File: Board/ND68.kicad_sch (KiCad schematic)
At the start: 210 parts

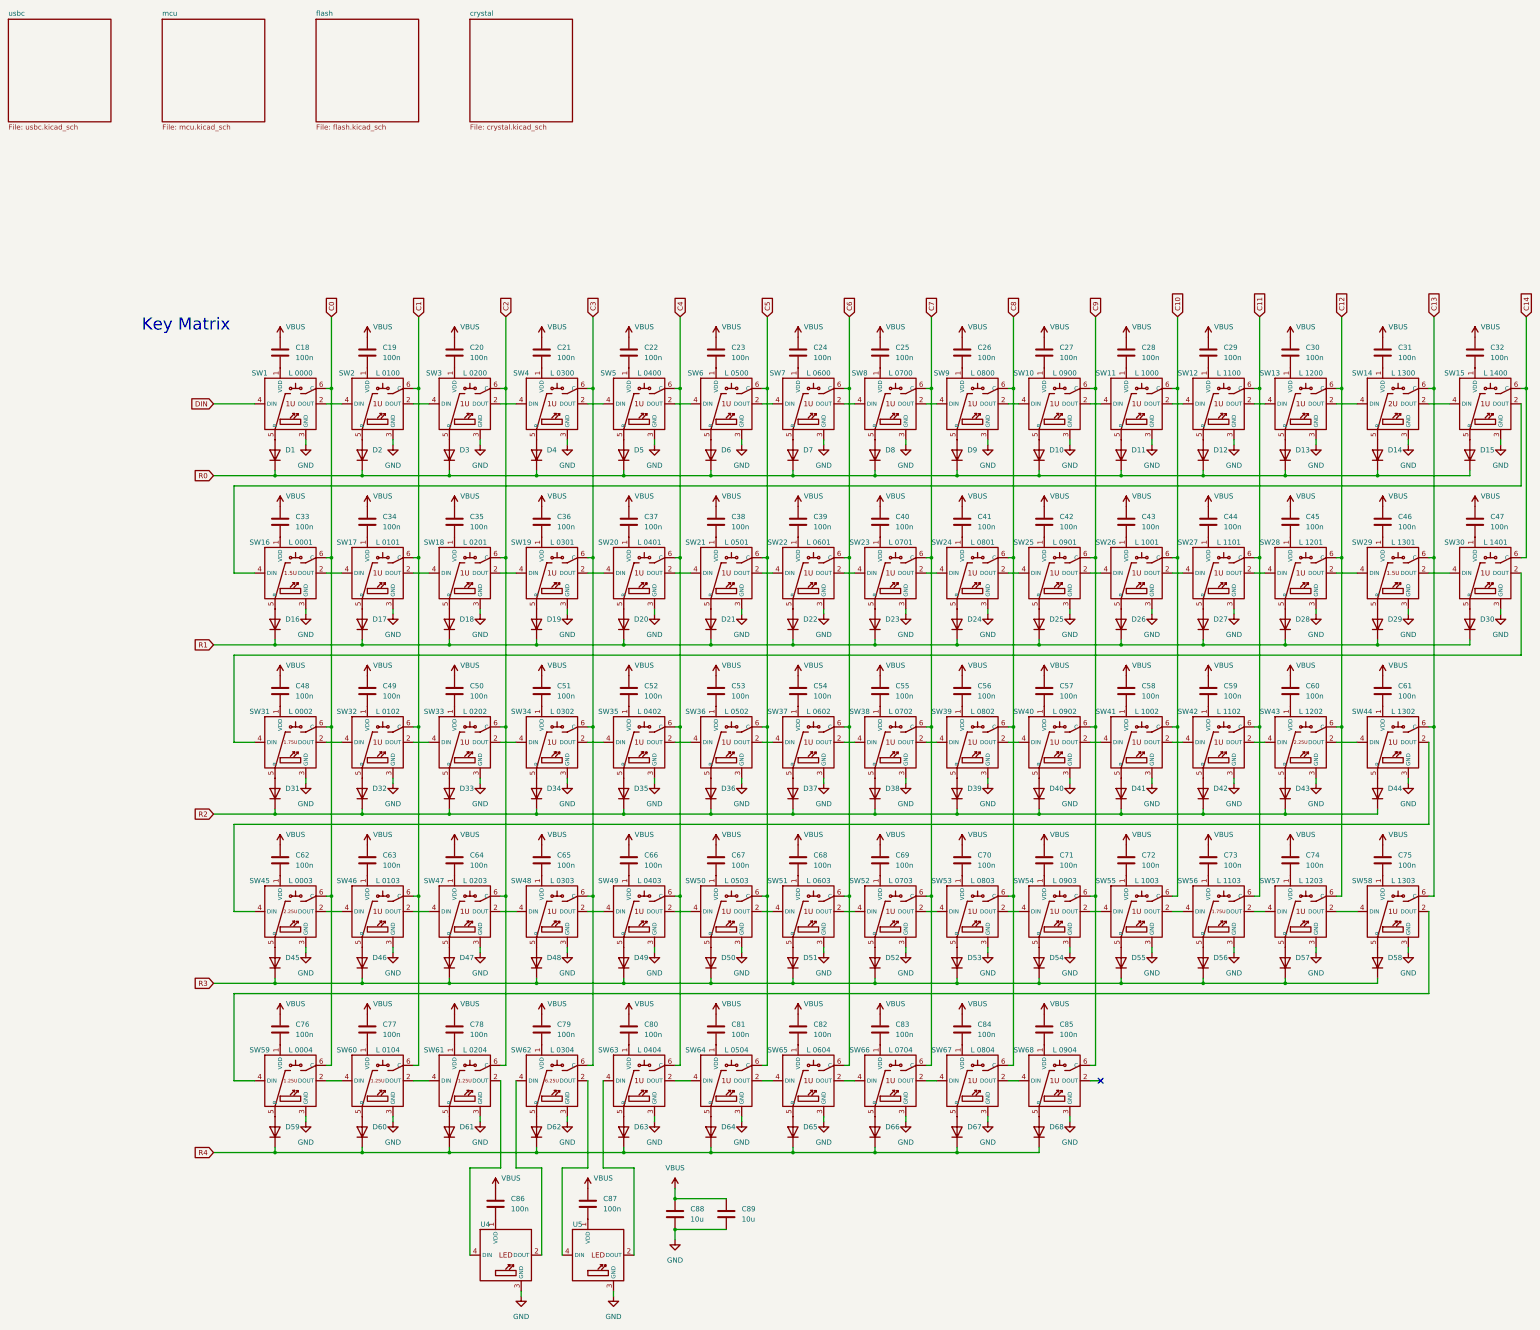
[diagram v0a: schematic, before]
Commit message: Rev 1 fix
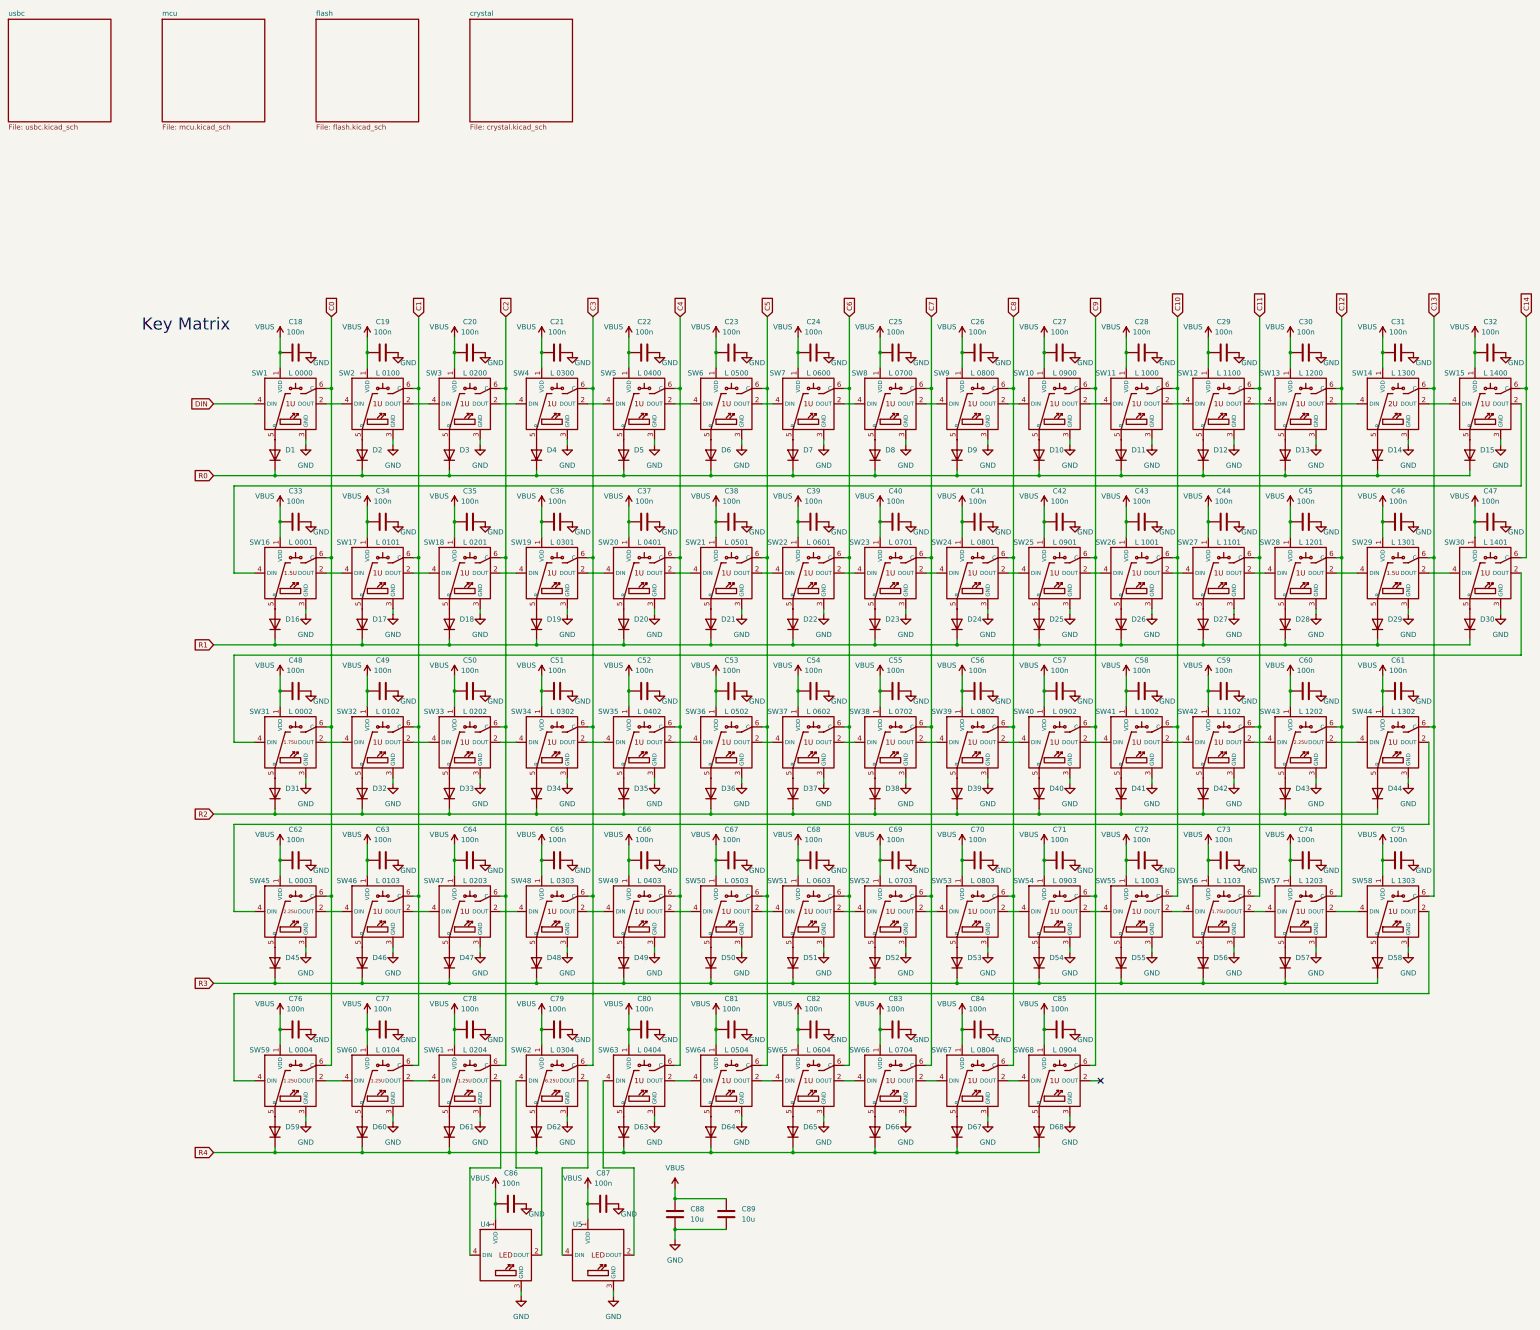
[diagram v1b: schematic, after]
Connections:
- net GND: now also C18.1, C19.2, C20.2, C21.2, C22.2, C23.2, C24.2, C25.2, C26.2, C27.2, C28.2, C29.2, C30.2, C31.2, C32.2, C33.2, C34.2, C35.2, C36.2, C37.2, C38.2, C39.2, C40.2, C41.2, C42.2, C43.2, C44.2, C45.2, C46.2, C47.2, C48.2, C49.2, C50.2, C51.2, C52.2, C53.2, C54.2, C55.2, C56.2, C57.2, C58.2, C59.2, C60.2, C61.2, C62.2, C63.2, C64.2, C65.2, C66.2, C67.2, C68.2, C69.2, C70.2, C71.2, C72.2, C73.2, C74.2, C75.2, C76.2, C77.2, C78.2, C79.2, C80.2, C81.2, C82.2, C83.2, C84.2, C85.2, C86.2, C87.2
- net VBUS: now also C18.2, SW1.1 (VDD), SW10.1 (VDD), SW11.1 (VDD), SW12.1 (VDD), SW13.1 (VDD), SW14.1 (VDD), SW15.1 (VDD), SW16.1 (VDD), SW17.1 (VDD), SW18.1 (VDD), SW19.1 (VDD), SW2.1 (VDD), SW20.1 (VDD), SW21.1 (VDD), SW22.1 (VDD), SW23.1 (VDD), SW24.1 (VDD), SW25.1 (VDD), SW26.1 (VDD), SW27.1 (VDD), SW28.1 (VDD), SW29.1 (VDD), SW3.1 (VDD), SW30.1 (VDD), SW31.1 (VDD), SW32.1 (VDD), SW33.1 (VDD), SW34.1 (VDD), SW35.1 (VDD), SW36.1 (VDD), SW37.1 (VDD), SW38.1 (VDD), SW39.1 (VDD), SW4.1 (VDD), SW40.1 (VDD), SW41.1 (VDD), SW42.1 (VDD), SW43.1 (VDD), SW44.1 (VDD), SW45.1 (VDD), SW46.1 (VDD), SW47.1 (VDD), SW48.1 (VDD), SW49.1 (VDD), SW5.1 (VDD), SW50.1 (VDD), SW51.1 (VDD), SW52.1 (VDD), SW53.1 (VDD), SW54.1 (VDD), SW55.1 (VDD), SW56.1 (VDD), SW57.1 (VDD), SW58.1 (VDD), SW59.1 (VDD), SW6.1 (VDD), SW60.1 (VDD), SW61.1 (VDD), SW62.1 (VDD), SW63.1 (VDD), SW64.1 (VDD), SW65.1 (VDD), SW66.1 (VDD), SW67.1 (VDD), SW68.1 (VDD), SW7.1 (VDD), SW8.1 (VDD), SW9.1 (VDD), U4.1 (VDD), U5.1 (VDD); no longer C18.1
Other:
- moved on the sheet: C18, C19, C20, C21, C22, C23, C24, C25, C26, C27, C28, C29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
